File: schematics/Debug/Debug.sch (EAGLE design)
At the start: 11 parts

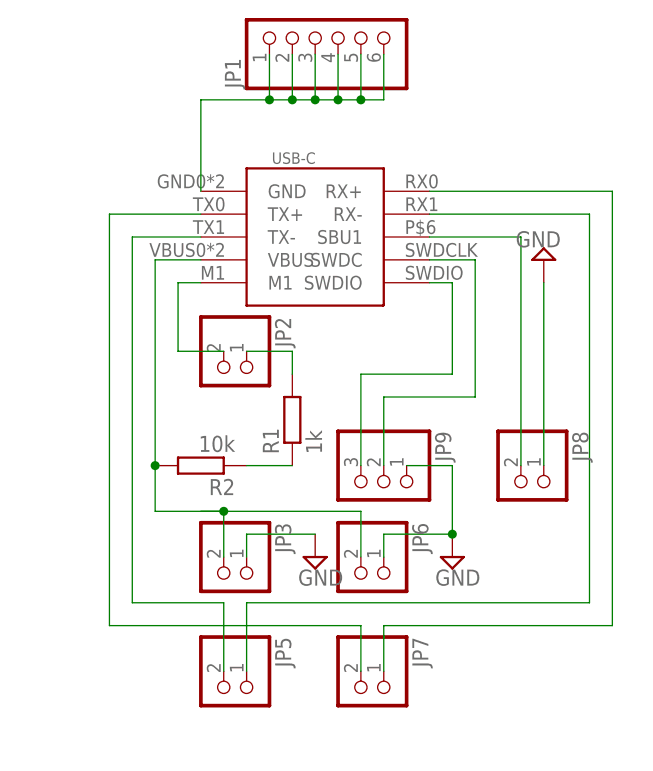
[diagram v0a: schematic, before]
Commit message: Кнопка на отладочной плате
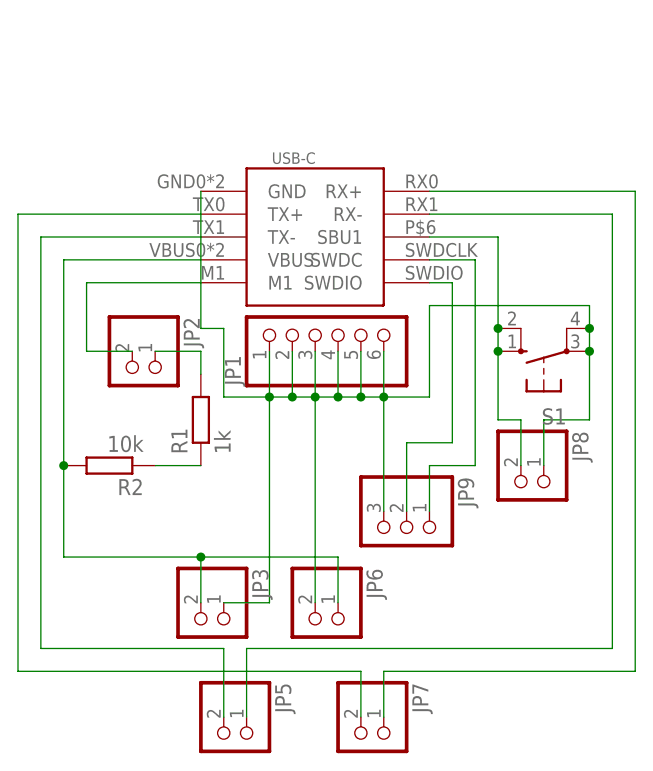
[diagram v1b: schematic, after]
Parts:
- added S1: (no value), switch-omron:10-XX
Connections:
- removed net GND: JP3.1, JP6.1, JP8.1, JP9.1
- removed net N$14: JP1.1, JP1.2, JP1.3, JP1.4, JP1.5, JP1.6, U$1.GND
- new net N$10: JP1.1, JP1.2, JP1.3, JP1.4, JP1.5, JP1.6, JP3.1, JP6.2, JP8.1, JP9.3, S1.P, S1.P1, U$1.GND
- net N$11: now also U$1.SWDIO; no longer U$1.SWDC
- net N$12: now also JP9.1, U$1.SWDC; no longer JP9.3, U$1.SWDIO
- net N$4: now also S1.S, S1.S1
- net N$6: now also JP6.1; no longer JP6.2
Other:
- moved on the sheet: JP1, JP2, JP3, JP5, JP6, JP7, JP9, R1, R2
